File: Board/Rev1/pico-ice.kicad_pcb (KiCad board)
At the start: 4 copper layers, 22.9 x 61 mm, 99 parts, among them J1 USB_C_Receptacle_USB2.0, J2 Conn_02x20_Odd_Even, J3 Conn_02x20_Odd_Even, J4 PB_SEL, Q1 2N7002, SW1 PTS820 J25K SMTR LFS, SW2 PTS820 J25K SMTR LFS, U1 CL9293A12L5M, U2 W25Q32JVSSIQ, U3 RP2040, U4 CL9293A33L5M, U5 APS6404L-3SQN-SN, U6 ICE40UP5K-SG48ITR, U8 W25Q32JVSSIQ, Y1 12 MHz

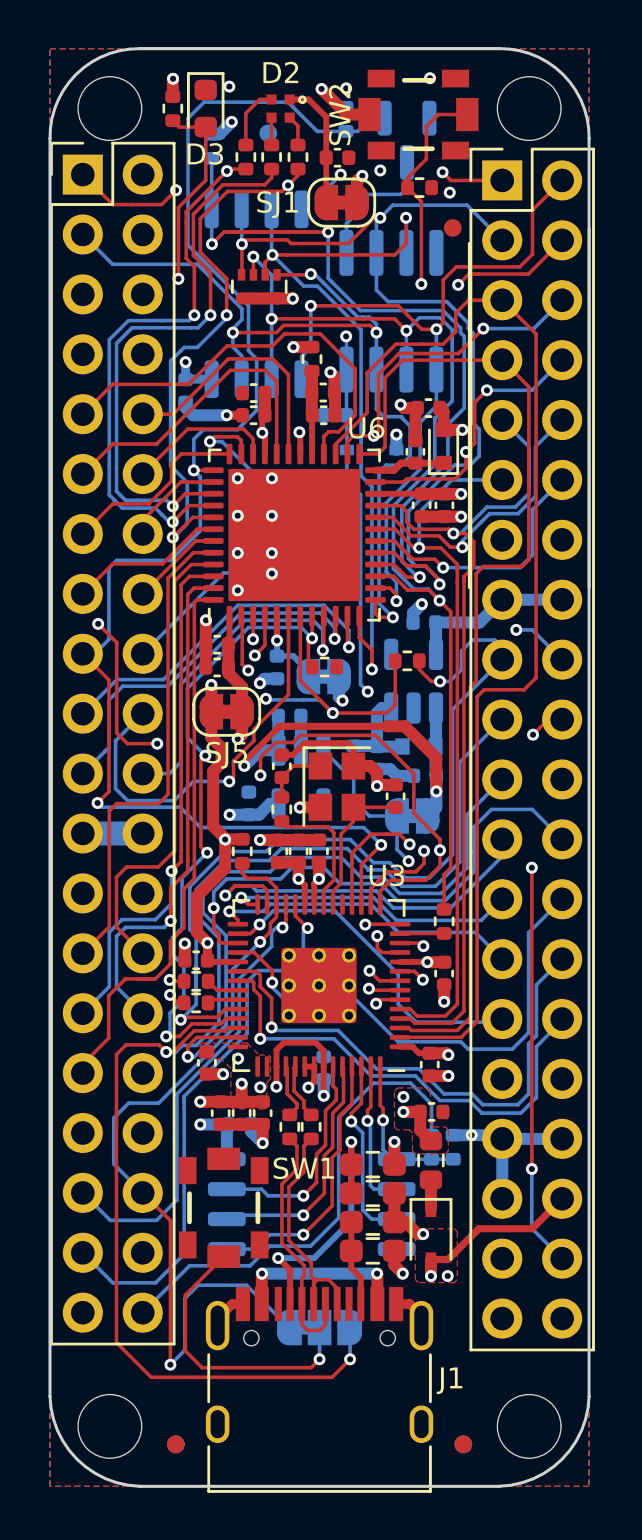
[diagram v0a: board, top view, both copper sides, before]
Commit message: Update pico-ice.kicad_pcb
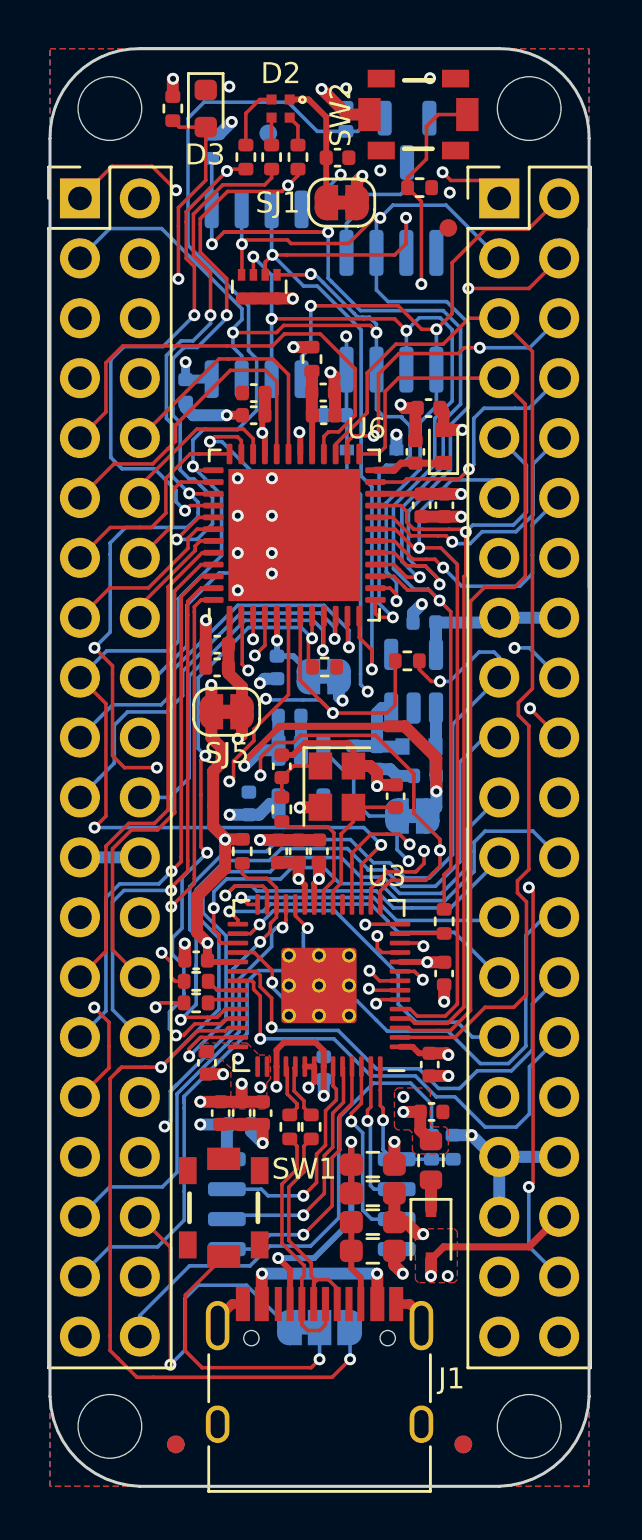
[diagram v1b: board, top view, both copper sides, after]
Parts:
- moved J2 1.02 mm to (62.2, 80.0)
- moved J3 0.77 mm to (80.0, 80.0)
- moved FID1 0.19 mm to (77.9, 81.3)
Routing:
- net /ICE_6: track 17.1 -> 12.6 mm
- net /ICE_4: track 29.8 -> 33.9 mm
- net /ICE_3: track 29.2 -> 33.2 mm
- net /LED_G: track 72.5 -> 70.0 mm
- net /PICO_PMOD_B3: track 22.2 -> 19.8 mm
- net /ICE_25: track 43.0 -> 41.0 mm
- net /~{ICE_RST}: track 53.2 -> 51.3 mm
- net /ICE_28: track 18.0 -> 19.7 mm
- net /ICE_35_G0: track 36.0 -> 37.6 mm
- net /LED_B: track 79.9 -> 78.2 mm
- net +3V3: track 60.3 -> 58.7 mm
- net /SRAM_SS: track 62.5 -> 64.1 mm
- net /ICE_27: track 48.2 -> 46.7 mm
- net /SWCLK: track 23.7 -> 22.3 mm
- net /ICE_SO: track 50.5 -> 49.2 mm
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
